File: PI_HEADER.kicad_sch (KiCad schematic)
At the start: 9 parts, among them J14 PRT-14017, J6 ADC_CONN

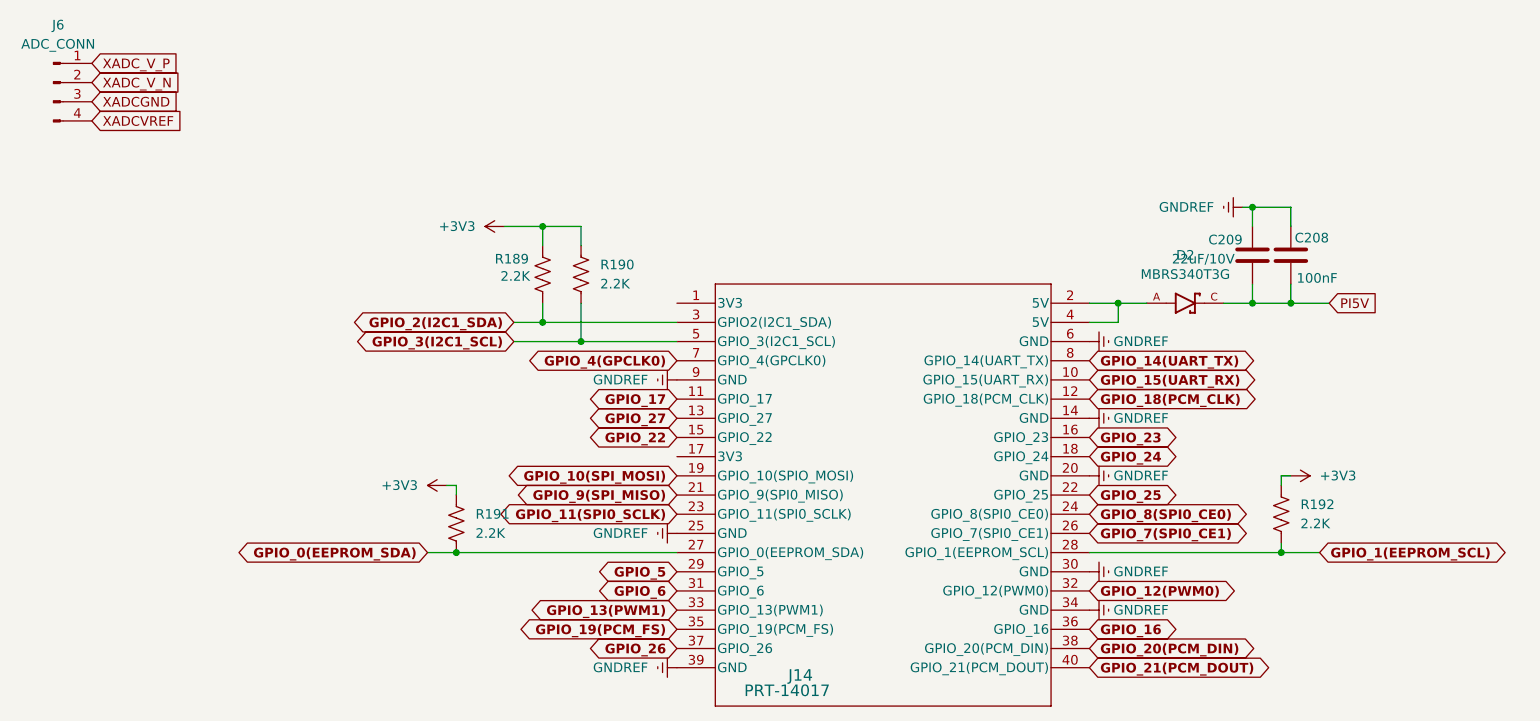
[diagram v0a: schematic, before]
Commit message: post -production rework
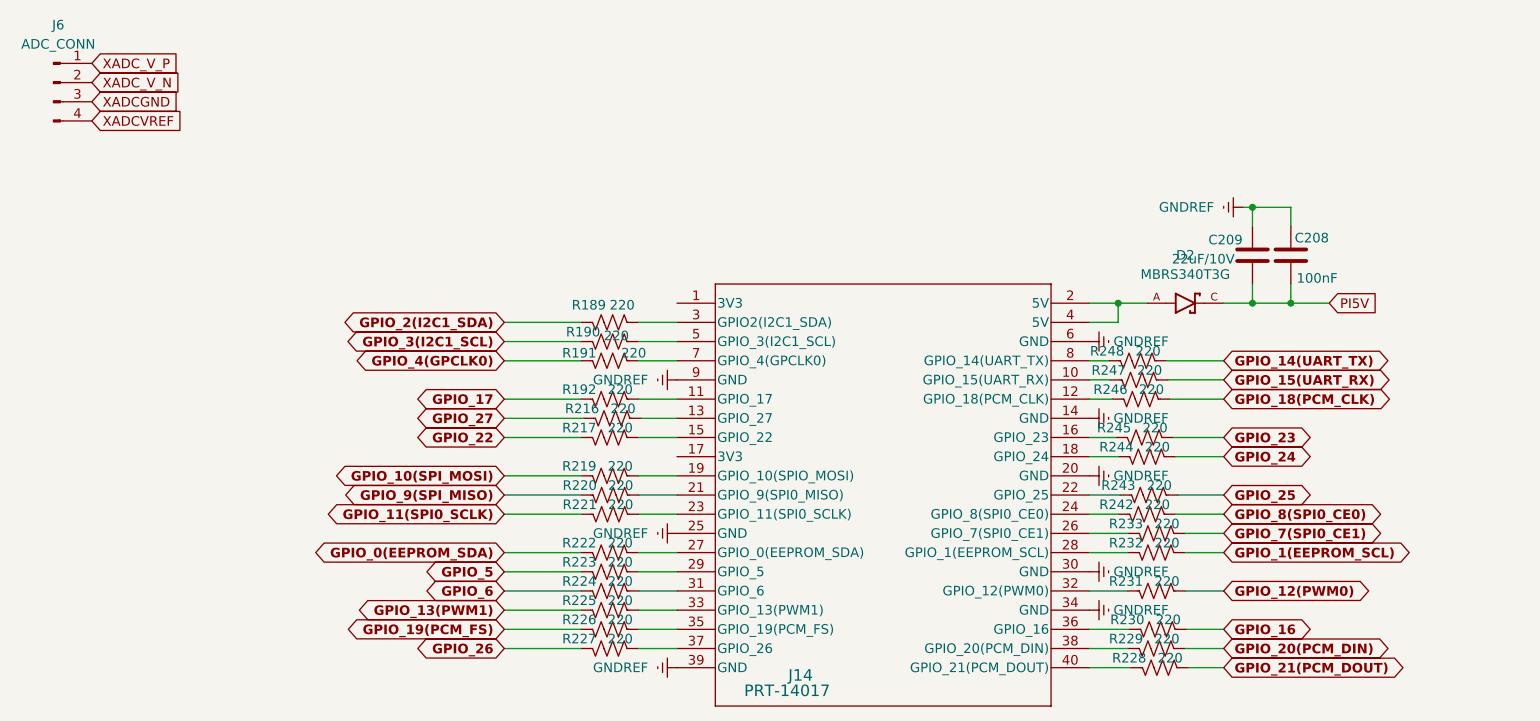
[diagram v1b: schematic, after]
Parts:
- added R216, R217, R219, R220, R221, R222, R223, R224, R225, R226, R227, R228, R229, R230, R231, R232, R233, R242, R243, R244, R245, R246, R247, R248: 220, footprints:R_0402, symbol Device:R_US
- R189, R190, R191, R192: value 2.2K -> 220; LCSC PN c114762 -> C112291
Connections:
- net GPIO_0(EEPROM_SDA): now also R222.1; no longer J14.27 (GPIO_0(EEPROM_SDA)), R191.1
- net GPIO_1(EEPROM_SCL): now also R232.2; no longer J14.28 (GPIO_1(EEPROM_SCL)), R192.1
- net GPIO_10(SPI_MOSI): now also R219.1; no longer J14.19 (GPIO_10(SPIO_MOSI))
- net GPIO_11(SPI0_SCLK): now also R221.1; no longer J14.23 (GPIO_11(SPI0_SCLK))
- net GPIO_12(PWM0): now also R231.2; no longer J14.32 (GPIO_12(PWM0))
- net GPIO_13(PWM1): now also R225.1; no longer J14.33 (GPIO_13(PWM1))
- net GPIO_14(UART_TX): now also R248.2; no longer J14.8 (GPIO_14(UART_TX))
- net GPIO_15(UART_RX): now also R247.2; no longer J14.10 (GPIO_15(UART_RX))
- net GPIO_16: now also R230.2; no longer J14.36 (GPIO_16)
- net GPIO_17: now also R192.1; no longer J14.11 (GPIO_17)
- net GPIO_18(PCM_CLK): now also R246.2; no longer J14.12 (GPIO_18(PCM_CLK))
- net GPIO_19(PCM_FS): now also R226.1; no longer J14.35 (GPIO_19(PCM_FS))
- net GPIO_2(I2C1_SDA): no longer J14.3 (GPIO2(I2C1_SDA))
- net GPIO_20(PCM_DIN): now also R229.2; no longer J14.38 (GPIO_20(PCM_DIN))
- net GPIO_21(PCM_DOUT): now also R228.2; no longer J14.40 (GPIO_21(PCM_DOUT))
- net GPIO_22: now also R217.1; no longer J14.15 (GPIO_22)
- net GPIO_23: now also R245.2; no longer J14.16 (GPIO_23)
- net GPIO_24: now also R244.2; no longer J14.18 (GPIO_24)
- net GPIO_25: now also R243.2; no longer J14.22 (GPIO_25)
- net GPIO_26: now also R227.1; no longer J14.37 (GPIO_26)
- net GPIO_27: now also R216.1; no longer J14.13 (GPIO_27)
- net GPIO_3(I2C1_SCL): no longer J14.5 (GPIO_3(I2C1_SCL))
- net GPIO_4(GPCLK0): now also R191.1; no longer J14.7 (GPIO_4(GPCLK0))
- net GPIO_5: now also R223.1; no longer J14.29 (GPIO_5)
- net GPIO_6: now also R224.1; no longer J14.31 (GPIO_6)
- net GPIO_7(SPI0_CE1): now also R233.2; no longer J14.26 (GPIO_7(SPI0_CE1))
- net GPIO_8(SPI0_CE0): now also R242.2; no longer J14.24 (GPIO_8(SPI0_CE0))
- net GPIO_9(SPI_MISO): now also R220.1; no longer J14.21 (GPIO_9(SPI0_MISO))
- removed net +3V3: R189.2, R190.2, R191.2, R192.2
- new net: J14.31 (GPIO_6), R224.2
- new net: J14.28 (GPIO_1(EEPROM_SCL)), R232.1
- new net: J14.16 (GPIO_23), R245.1
- new net: J14.19 (GPIO_10(SPIO_MOSI)), R219.2
- new net: J14.27 (GPIO_0(EEPROM_SDA)), R222.2
- new net: J14.36 (GPIO_16), R230.1
- new net: J14.8 (GPIO_14(UART_TX)), R248.1
- new net: J14.37 (GPIO_26), R227.2
- new net: J14.18 (GPIO_24), R244.1
- new net: J14.15 (GPIO_22), R217.2
- new net: J14.10 (GPIO_15(UART_RX)), R247.1
- new net: J14.11 (GPIO_17), R192.2
- new net: J14.12 (GPIO_18(PCM_CLK)), R246.1
- new net: J14.13 (GPIO_27), R216.2
- new net: J14.21 (GPIO_9(SPI0_MISO)), R220.2
- new net: J14.22 (GPIO_25), R243.1
- new net: J14.23 (GPIO_11(SPI0_SCLK)), R221.2
- new net: J14.24 (GPIO_8(SPI0_CE0)), R242.1
- new net: J14.26 (GPIO_7(SPI0_CE1)), R233.1
- new net: J14.29 (GPIO_5), R223.2
- new net: J14.3 (GPIO2(I2C1_SDA)), R189.2
- new net: J14.32 (GPIO_12(PWM0)), R231.1
- new net: J14.33 (GPIO_13(PWM1)), R225.2
- new net: J14.35 (GPIO_19(PCM_FS)), R226.2
- new net: J14.38 (GPIO_20(PCM_DIN)), R229.1
- new net: J14.40 (GPIO_21(PCM_DOUT)), R228.1
- new net: J14.5 (GPIO_3(I2C1_SCL)), R190.2
- new net: J14.7 (GPIO_4(GPCLK0)), R191.2
